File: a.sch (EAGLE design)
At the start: 31 parts, among them CON1 PINHEAD_1X04-2.54, CON3 PINHEAD_1X07-2.54, SW1 TACT_SWITCH-1-1825910-4, SW2 TACT_SWITCH-1-1825910-4, X3 PINHEAD_1X06-2-MALE, X4 PINHEAD_2X03-PTH-2.54

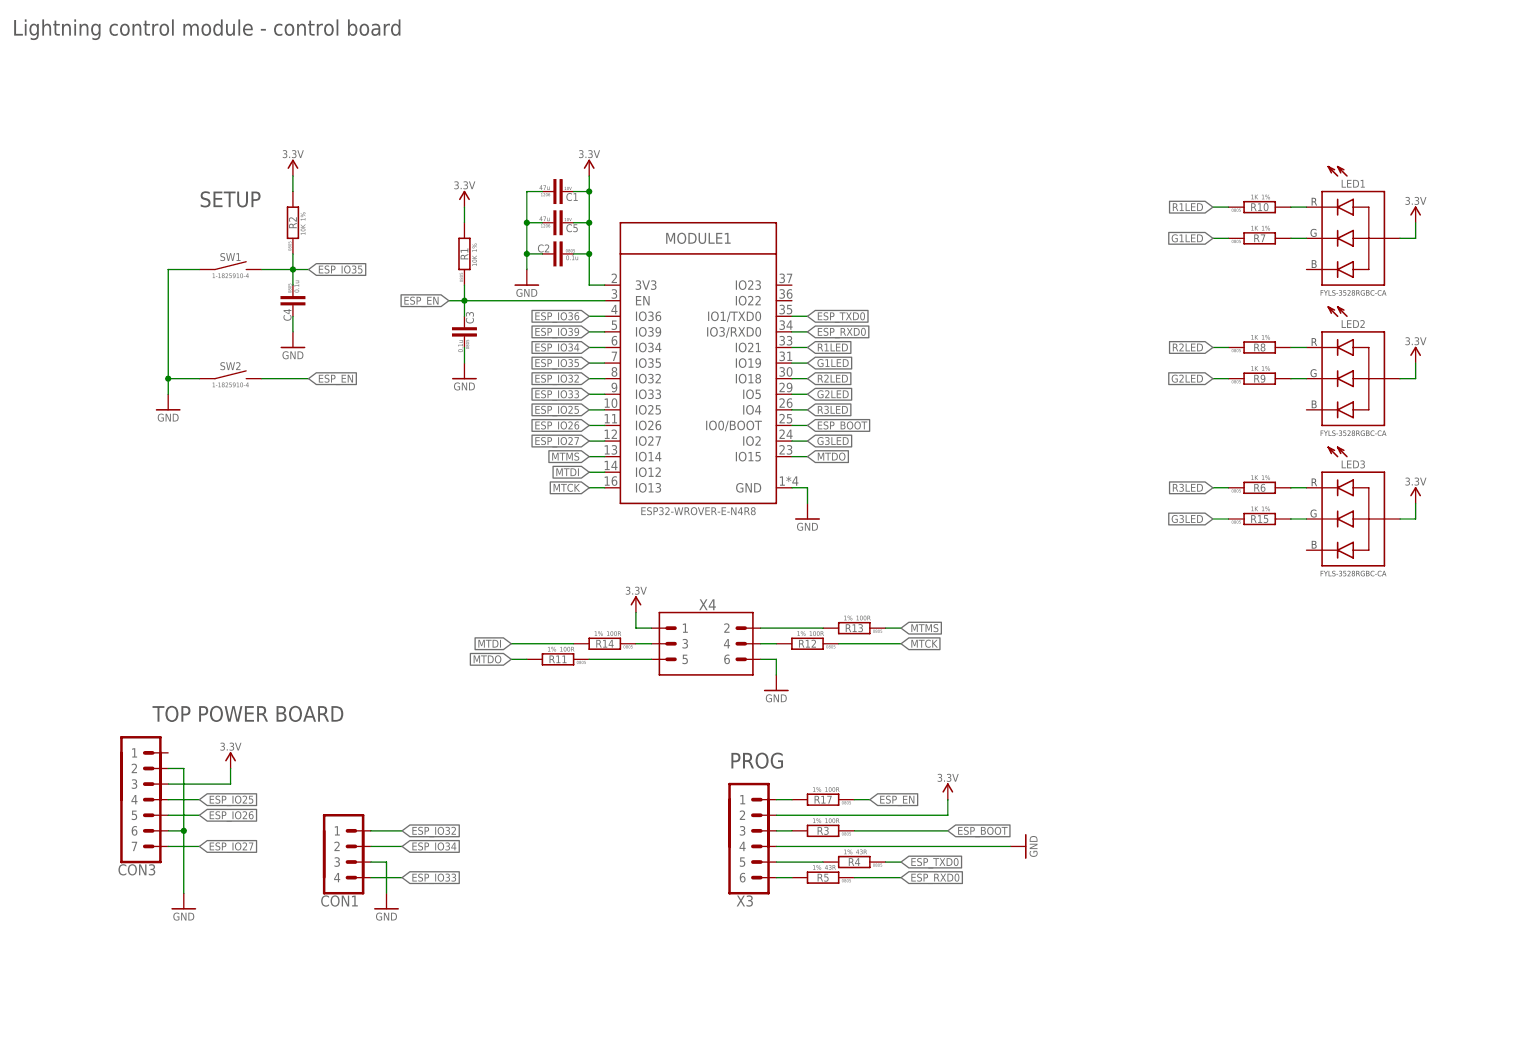
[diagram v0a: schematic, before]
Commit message: A pcb updated
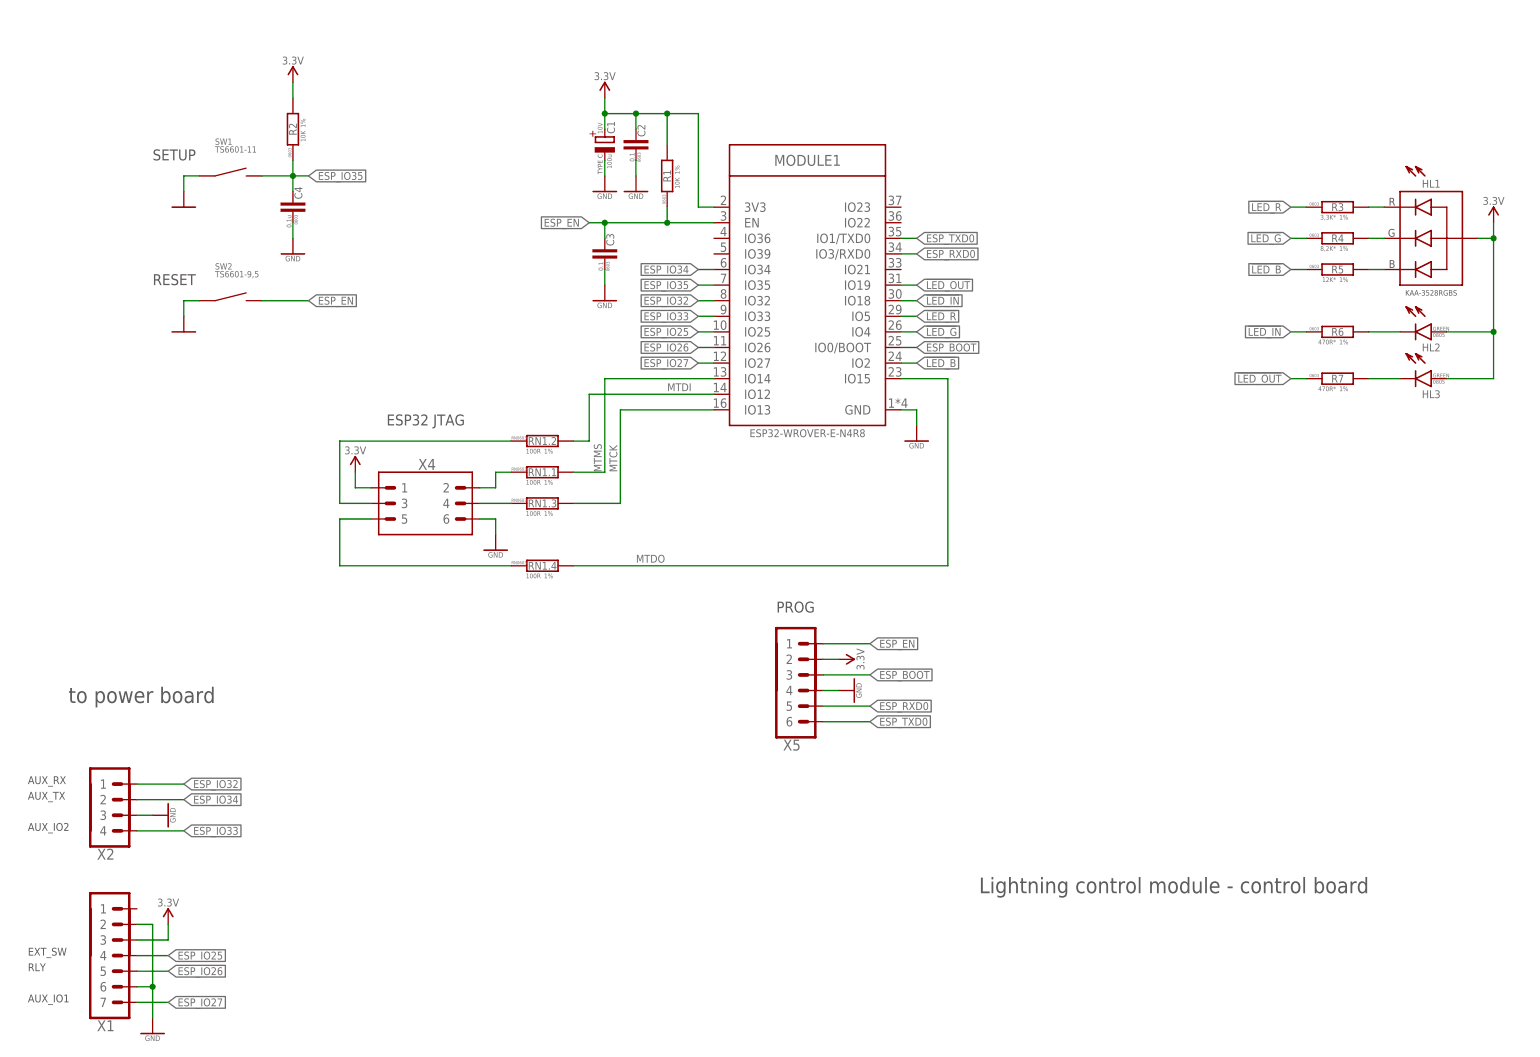
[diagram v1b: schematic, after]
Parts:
- removed C5: 47u, rc:C-1206
- removed CON1: PINHEAD_1X04-2.54, pinhead:PINHEAD_1X04-2.54
- removed CON3: PINHEAD_1X07-2.54, pinhead:PINHEAD_1X07-2.54
- removed LED1, LED2, LED3: LED_RGB-3528, rc:LED_RGB-3528
- removed R10, R15, R8, R9: 1K, rc:R-1%-0805
- removed R11, R12, R13, R14, R17: 100R, rc:R-1%-0805
- removed X3: PINHEAD_1X06-2-MALE, pinhead:PINHEAD_1X06-2-MALE
- added HL1: LED_RGB-KAA-3528RGBS, rc:LED_RGB-KAA-3528RGBS
- added HL2, HL3: LED-0805, rc:LED-0805
- added RN1: 100R, rc:RN-1%-0603
- added X1: PINHEAD_1X07-2.54, pinhead:PINHEAD_1X07-2.54
- added X2: PINHEAD_1X04-2.54, pinhead:PINHEAD_1X04-2.54
- added X5: PINHEAD_1X06-2-MALE, pinhead:PINHEAD_1X06-2-MALE
- C1: value 47u -> 100u; device rc:C-1206 -> rc:CPOL-TANT-TYPE-C
- C2, C3: value 0.1u -> 0.1; device rc:C-0805 -> rc:C-0603
- C4: device rc:C-0805 -> rc:C-0603
- R1, R2: device rc:R-1%-0805 -> rc:R-1%-0603
- R3: value 100R -> 3,3K*; device rc:R-1%-0805 -> rc:R-1%-0603
- R4: value 43R -> 8,2K*; device rc:R-1%-0805 -> rc:R-1%-0603
- R5: value 43R -> 12K*; device rc:R-1%-0805 -> rc:R-1%-0603
- R6, R7: value 1K -> 470R*; device rc:R-1%-0805 -> rc:R-1%-0603
- SW1: value TACT_SWITCH-1-1825910-4 -> TS6601-11; device mechanical:TACT_SWITCH-1-1825910-4 -> mechanical:TACT_SWITCH-6X6-PTH
- SW2: value TACT_SWITCH-1-1825910-4 -> TS6601-9,5; device mechanical:TACT_SWITCH-1-1825910-4 -> mechanical:TACT_SWITCH-6X6-PTH
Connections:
- net G1LED renamed !LED_OUT
- removed net ESP_IO36: MODULE1.IO36
- removed net ESP_IO39: MODULE1.IO39
- removed net G2LED: MODULE1.IO5, R9.1
- removed net G3LED: MODULE1.IO2, R15.1
- removed net N$10: LED3.R, R6.2
- removed net N$11: LED3.G, R15.2
- removed net N$14: R14.1, X4.3
- removed net N$15: R11.1, X4.5
- removed net N$17: R17.2, X3.1
- removed net N$3: R5.2, X3.6
- removed net N$5: R3.2, X3.3
- removed net N$6: R12.2, X4.4
- removed net N$7: LED1.R, R10.2
- removed net N$9: LED2.G, R9.2
- removed net R1LED: MODULE1.IO21, R10.1
- removed net R2LED: MODULE1.IO18, R8.1
- removed net R3LED: MODULE1.IO4, R6.1
- new net !LED_B: MODULE1.IO2, R5.1
- new net !LED_G: MODULE1.IO4, R4.1
- new net !LED_IN: MODULE1.IO18, R6.1
- new net !LED_R: MODULE1.IO5, R3.1
- new net N$124: RN1.4.1, X4.5
- new net N$150: RN1.1.1, X4.2
- new net N$18: HL3.C, R7.2
- new net N$213: RN1.2.1, X4.3
- new net N$216: RN1.3.1, X4.4
- net ESP_BOOT: now also X5.3; no longer R3.1
- net ESP_EN: now also X5.1; no longer R17.1
- net ESP_IO25: now also X1.4; no longer CON3.4
- net ESP_IO26: now also X1.5; no longer CON3.5
- net ESP_IO27: now also X1.7; no longer CON3.7
- net ESP_IO32: now also X2.1; no longer CON1.1
- net ESP_IO33: now also X2.4; no longer CON1.4
- net ESP_IO34: now also X2.2; no longer CON1.2
- net ESP_IO35: now also C4.2; no longer C4.1
- net ESP_RXD0: now also X5.5; no longer R5.1
- net ESP_TXD0: now also X5.6; no longer R4.1
- net GND: now also C1.-, C2.1, C4.1, X1.2, X1.6, X2.3, X5.4; no longer C1.1, C2.2, C4.2, C5.1, CON1.3, CON3.2, CON3.6, X3.4
- net MTCK: now also RN1.3.2; no longer R12.1
- net MTDI: now also RN1.2.2; no longer R14.2
- net MTDO: now also RN1.4.2; no longer R11.2
- net MTMS: now also RN1.1.2; no longer R13.1
- net N$1: now also HL1.B, R5.2; no longer LED2.R, R8.2
- net N$2: now also HL1.G, R4.2; no longer R13.2, X4.2
- net N$4: now also HL1.R, R3.2; no longer R4.2, X3.5
- net N$8: now also HL2.C, R6.2; no longer LED1.G, R7.2
- net VDD_3V3: now also C1.+, C2.2, HL1.A, HL2.A, HL3.A, X1.3, X5.2; no longer C1.2, C2.1, C5.2, CON3.3, LED1.A, LED2.A, LED3.A, X3.2
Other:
- note added: "AUX_IO1"
- note added: "AUX_IO2"
- note added: "AUX_RX"
- note added: "AUX_TX"
- note added: "ESP32 JTAG"
- note added: "EXT_SW"
- note added: "RESET"
- note added: "RLY"
- note added: "to power board"
- note removed: "TOP POWER BOARD"
- moved on the sheet: C2, C3, C4, MODULE1, R1, R2, R3, R4, R5, R6, R7, SW1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

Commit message: Import
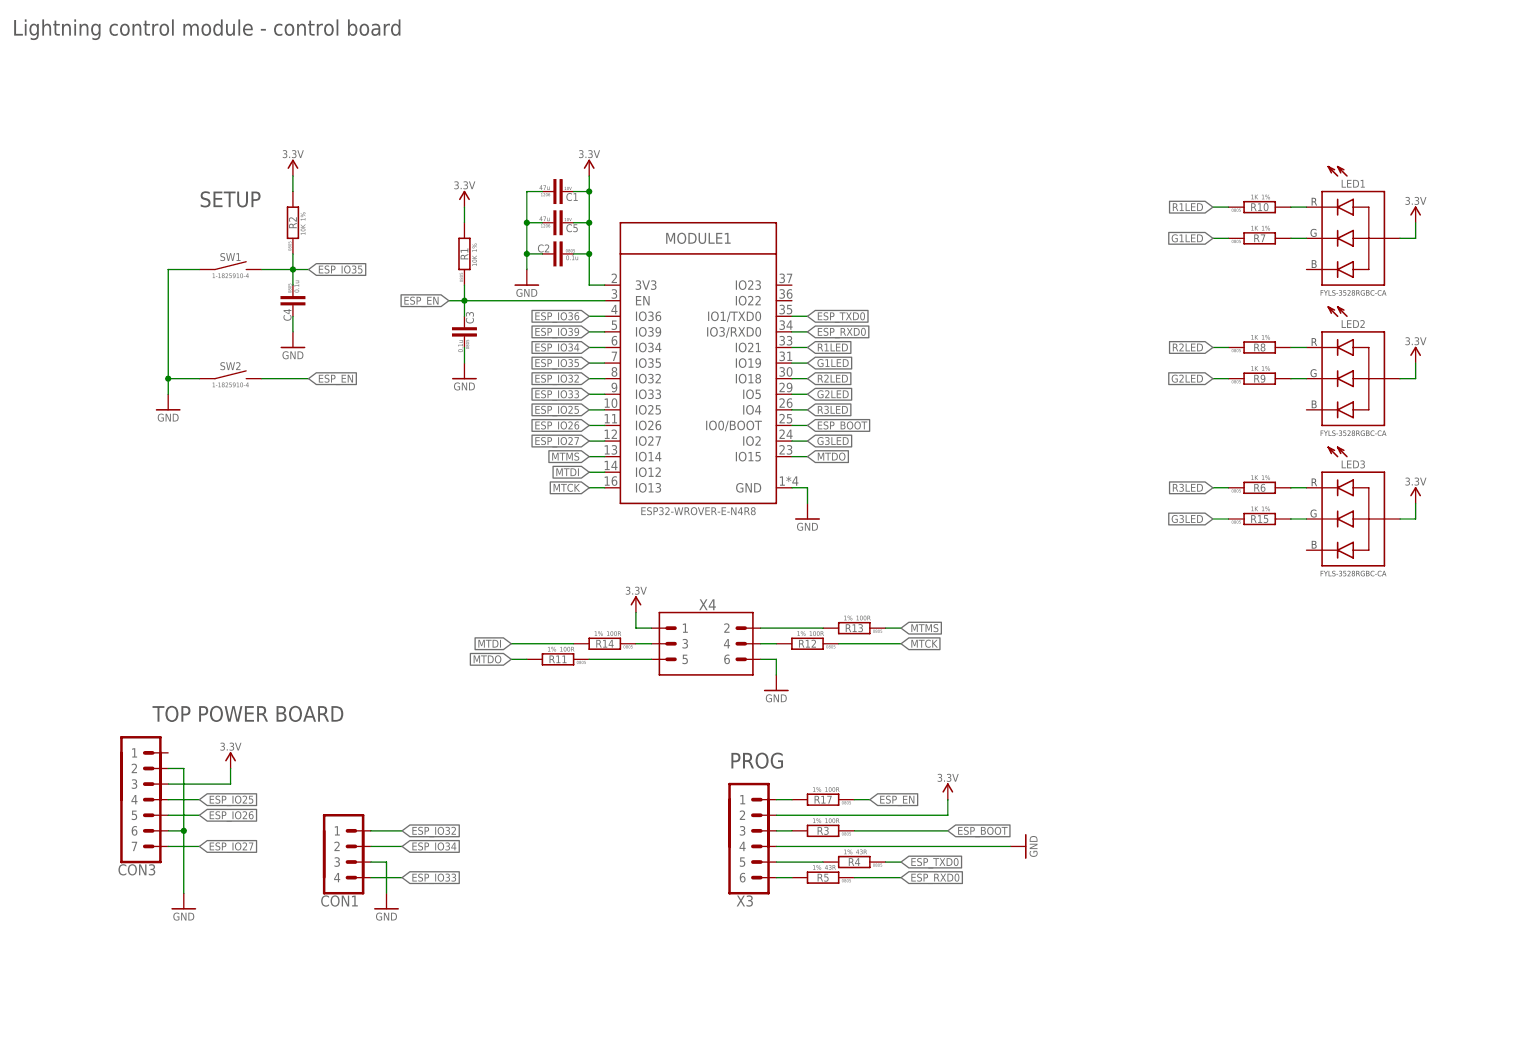
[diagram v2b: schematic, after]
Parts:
- removed HL1: LED_RGB-KAA-3528RGBS, rc:LED_RGB-KAA-3528RGBS
- removed HL2, HL3: LED-0805, rc:LED-0805
- removed RN1: 100R, rc:RN-1%-0603
- removed X1: PINHEAD_1X07-2.54, pinhead:PINHEAD_1X07-2.54
- removed X2: PINHEAD_1X04-2.54, pinhead:PINHEAD_1X04-2.54
- removed X5: PINHEAD_1X06-2-MALE, pinhead:PINHEAD_1X06-2-MALE
- added C5: 47u, rc:C-1206
- added CON1: PINHEAD_1X04-2.54, pinhead:PINHEAD_1X04-2.54
- added CON3: PINHEAD_1X07-2.54, pinhead:PINHEAD_1X07-2.54
- added LED1, LED2, LED3: LED_RGB-3528, rc:LED_RGB-3528
- added R10, R15, R8, R9: 1K, rc:R-1%-0805
- added R11, R12, R13, R14, R17: 100R, rc:R-1%-0805
- added X3: PINHEAD_1X06-2-MALE, pinhead:PINHEAD_1X06-2-MALE
- C1: value 100u -> 47u; device rc:CPOL-TANT-TYPE-C -> rc:C-1206
- C2, C3: value 0.1 -> 0.1u; device rc:C-0603 -> rc:C-0805
- C4: device rc:C-0603 -> rc:C-0805
- R1, R2: device rc:R-1%-0603 -> rc:R-1%-0805
- R3: value 3,3K* -> 100R; device rc:R-1%-0603 -> rc:R-1%-0805
- R4: value 8,2K* -> 43R; device rc:R-1%-0603 -> rc:R-1%-0805
- R5: value 12K* -> 43R; device rc:R-1%-0603 -> rc:R-1%-0805
- R6, R7: value 470R* -> 1K; device rc:R-1%-0603 -> rc:R-1%-0805
- SW1: value TS6601-11 -> TACT_SWITCH-1-1825910-4; device mechanical:TACT_SWITCH-6X6-PTH -> mechanical:TACT_SWITCH-1-1825910-4
- SW2: value TS6601-9,5 -> TACT_SWITCH-1-1825910-4; device mechanical:TACT_SWITCH-6X6-PTH -> mechanical:TACT_SWITCH-1-1825910-4
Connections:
- net !LED_OUT renamed G1LED
- removed net !LED_B: MODULE1.IO2, R5.1
- removed net !LED_G: MODULE1.IO4, R4.1
- removed net !LED_IN: MODULE1.IO18, R6.1
- removed net !LED_R: MODULE1.IO5, R3.1
- removed net N$124: RN1.4.1, X4.5
- removed net N$150: RN1.1.1, X4.2
- removed net N$18: HL3.C, R7.2
- removed net N$213: RN1.2.1, X4.3
- removed net N$216: RN1.3.1, X4.4
- new net ESP_IO36: MODULE1.IO36
- new net ESP_IO39: MODULE1.IO39
- new net G2LED: MODULE1.IO5, R9.1
- new net G3LED: MODULE1.IO2, R15.1
- new net N$10: LED3.R, R6.2
- new net N$11: LED3.G, R15.2
- new net N$14: R14.1, X4.3
- new net N$15: R11.1, X4.5
- new net N$17: R17.2, X3.1
- new net N$3: R5.2, X3.6
- new net N$5: R3.2, X3.3
- new net N$6: R12.2, X4.4
- new net N$7: LED1.R, R10.2
- new net N$9: LED2.G, R9.2
- new net R1LED: MODULE1.IO21, R10.1
- new net R2LED: MODULE1.IO18, R8.1
- new net R3LED: MODULE1.IO4, R6.1
- net ESP_BOOT: now also R3.1; no longer X5.3
- net ESP_EN: now also R17.1; no longer X5.1
- net ESP_IO25: now also CON3.4; no longer X1.4
- net ESP_IO26: now also CON3.5; no longer X1.5
- net ESP_IO27: now also CON3.7; no longer X1.7
- net ESP_IO32: now also CON1.1; no longer X2.1
- net ESP_IO33: now also CON1.4; no longer X2.4
- net ESP_IO34: now also CON1.2; no longer X2.2
- net ESP_IO35: now also C4.1; no longer C4.2
- net ESP_RXD0: now also R5.1; no longer X5.5
- net ESP_TXD0: now also R4.1; no longer X5.6
- net GND: now also C1.1, C2.2, C4.2, C5.1, CON1.3, CON3.2, CON3.6, X3.4; no longer C1.-, C2.1, C4.1, X1.2, X1.6, X2.3, X5.4
- net MTCK: now also R12.1; no longer RN1.3.2
- net MTDI: now also R14.2; no longer RN1.2.2
- net MTDO: now also R11.2; no longer RN1.4.2
- net MTMS: now also R13.1; no longer RN1.1.2
- net N$1: now also LED2.R, R8.2; no longer HL1.B, R5.2
- net N$2: now also R13.2, X4.2; no longer HL1.G, R4.2
- net N$4: now also R4.2, X3.5; no longer HL1.R, R3.2
- net N$8: now also LED1.G, R7.2; no longer HL2.C, R6.2
- net VDD_3V3: now also C1.2, C2.1, C5.2, CON3.3, LED1.A, LED2.A, LED3.A, X3.2; no longer C1.+, C2.2, HL1.A, HL2.A, HL3.A, X1.3, X5.2
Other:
- note added: "TOP POWER BOARD"
- note removed: "AUX_IO1"
- note removed: "AUX_IO2"
- note removed: "AUX_RX"
- note removed: "AUX_TX"
- note removed: "ESP32 JTAG"
- note removed: "EXT_SW"
- note removed: "RESET"
- note removed: "RLY"
- note removed: "to power board"
- moved on the sheet: C2, C3, C4, MODULE1, R1, R2, R3, R4, R5, R6, R7, SW1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
